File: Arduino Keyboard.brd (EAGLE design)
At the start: 168.9 x 50.8 mm, 26 parts, among them SW1 CHERRY-MXSTANDARD, SW10 CHERRY-MXSTANDARD, SW11 CHERRY-MXSTANDARD, SW12 CHERRY-MXSTANDARD, SW13 CHERRY-MXSTANDARD, SW14 CHERRY-MXSTANDARD, SW15 CHERRY-MXSTANDARD, SW16 CHERRY-MXSTANDARD, SW17 CHERRY-MXSTANDARD, SW18 CHERRY-MXSTANDARD, SW19 CHERRY-MXSTANDARD, SW2 CHERRY-MXSTANDARD, SW20 CHERRY-MXSTANDARD, SW3 CHERRY-MXSTANDARD, SW4 CHERRY-MXSTANDARD, SW5 CHERRY-MXSTANDARD, SW6 CHERRY-MXSTANDARD, SW7 CHERRY-MXSTANDARD, SW8 CHERRY-MXSTANDARD, SW9 CHERRY-MXSTANDARD

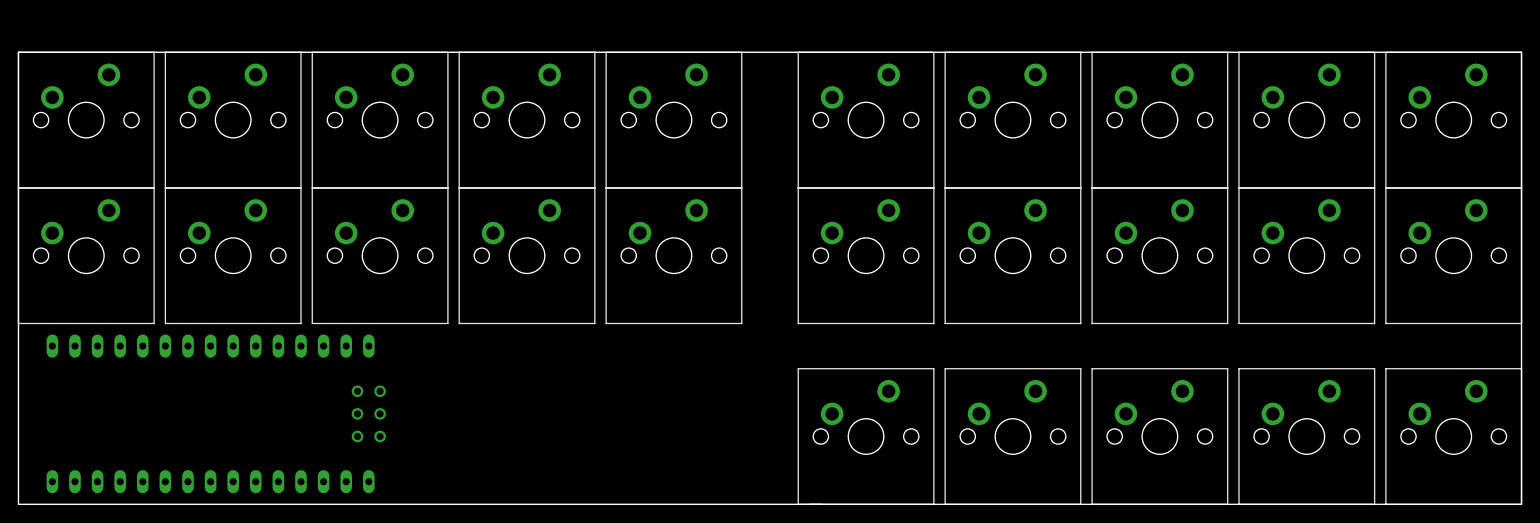
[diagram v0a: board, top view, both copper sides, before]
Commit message: Version 0.4
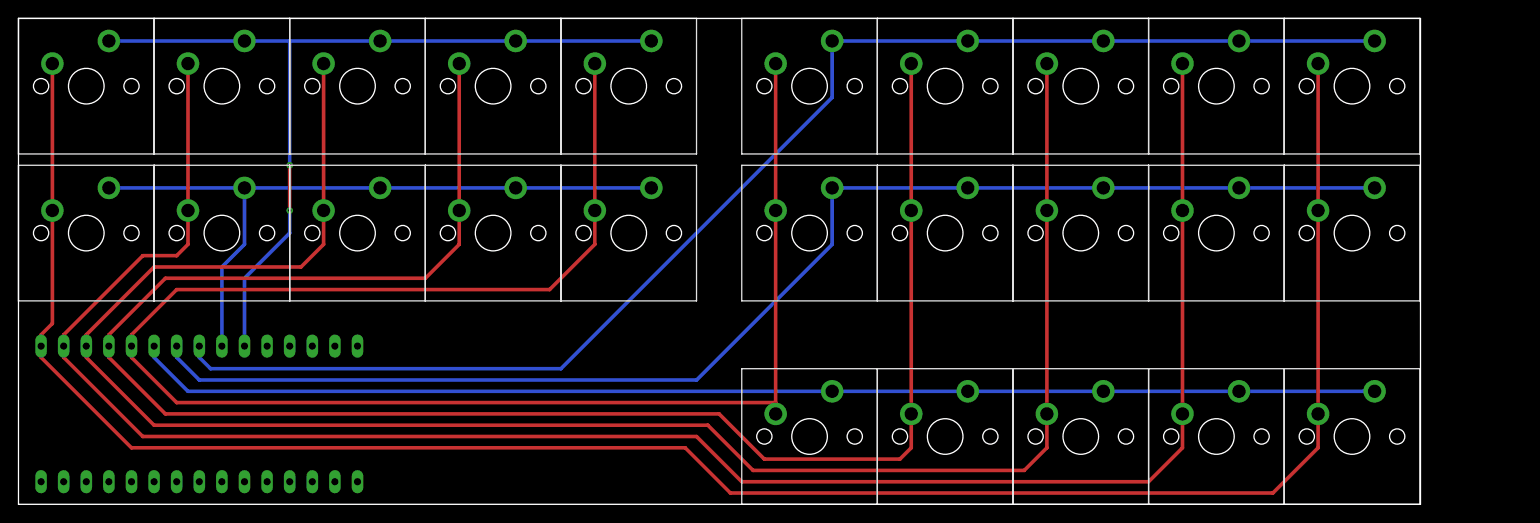
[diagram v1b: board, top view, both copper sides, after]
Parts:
- U$1: device Arduino-clone:NANO -> Arduino-clone_2:NANO
- moved SWS5 66.1 mm to (7.62, 47.0)
- moved SW20 66.1 mm to (7.62, 30.5)
- moved SW11 56.0 mm to (88.9, 47.0)
- moved SW6 55.9 mm to (88.9, 30.5)
- moved SW1 55.9 mm to (88.9, 7.62)
- moved SW14 39.6 mm to (134.6, 47.0)
- moved SW9 39.5 mm to (134.6, 30.5)
- moved SW4 39.4 mm to (134.6, 7.62)
- moved SW12 24.4 mm to (104.1, 47.0)
- moved SW7 24.3 mm to (104.1, 30.5)
- moved SW2 24.1 mm to (104.1, 7.62)
- moved SWS4 15.7 mm to (22.9, 47.0)
- moved SW19 15.5 mm to (22.9, 30.5)
- moved SWS3 14.5 mm to (38.1, 47.0)
- moved SW18 14.2 mm to (38.1, 30.5)
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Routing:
- net N$10: track 0.00 -> 228.7 mm
- net N$9: track 0.00 -> 217.3 mm
- net N$8: track 0.00 -> 211.2 mm
- net N$7: track 0.00 -> 205.0 mm
- net N$6: track 0.00 -> 193.0 mm
- net N$3: track 0.00 -> 152.9 mm
- net N$4: track 0.00 -> 149.6 mm
- net N$5: track 0.00 -> 141.3 mm
- net N$1: track 0.00 -> 97.4 mm, vias 0 -> 2
- net N$2: track 0.00 -> 79.8 mm
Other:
- board size 168.9 x 50.8 mm -> 157.6 x 54.6 mm
